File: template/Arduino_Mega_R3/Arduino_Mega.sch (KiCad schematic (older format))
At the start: 7 parts, among them P1 Digital, P2 Power, P3 Analog, P4 Analog, P5 PWM, P6 PWM, P7 Communication

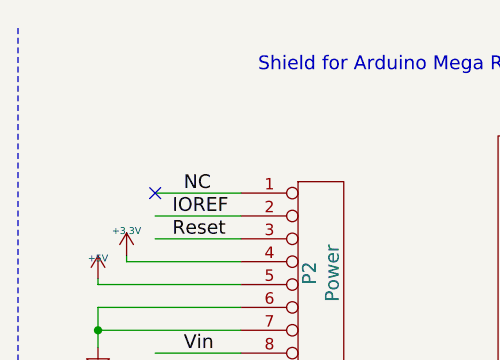
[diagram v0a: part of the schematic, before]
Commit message: correction holes
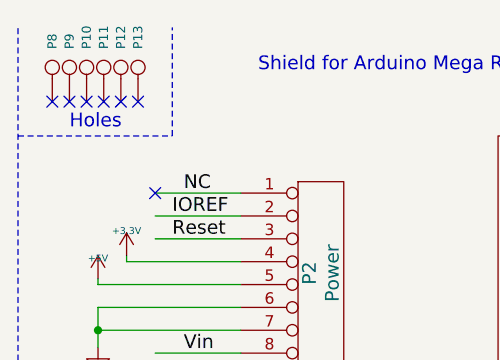
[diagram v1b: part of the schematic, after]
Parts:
- added P10, P11, P12, P13, P8, P9: CONN_1, Connect:1pin, symbol CONN_1
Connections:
- no-connect marks 1 -> 7
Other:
- note added: "Holes"
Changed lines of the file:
@@
 Wire Notes Line
 	7900 6300 7900 475
+$Comp
+L CONN_1 P8
+U 1 1 551BBA20
+P 8050 650
+F 0 "P8" H 8130 650 40  0000 L CNN
+F 1 "CONN_1" H 8050 705 30  0001 C CNN
+F 2 "Connect:1pin" H 8050 650 60  0001 C CNN
+F 3 "" H 8050 650 60  0000 C CNN
+	1    8050 650
+	0    -1   -1   0
+$EndComp
+$Comp
+L CONN_1 P9
+U 1 1 551BBB85
+P 8125 650
+F 0 "P9" H 8205 650 40  0000 L CNN
+F 1 "CONN_1" H 8125 705 30  0001 C CNN
+F 2 "Connect:1pin" H 8125 650 60  0001 C CNN
+F 3 "" H 8125 650 60  0000 C CNN
+	1    8125 650
+	0    -1   -1   0
+$EndComp
+$Comp
+L CONN_1 P10
+U 1 1 551BBBAB
+P 8200 650
+F 0 "P10" H 8280 650 40  0000 L CNN
+F 1 "CONN_1" H 8200 705 30  0001 C CNN
+F 2 "Connect:1pin" H 8200 650 60  0001 C CNN
+F 3 "" H 8200 650 60  0000 C CNN
+	1    8200 650
+	0    -1   -1   0
+$EndComp
+$Comp
+L CONN_1 P11
+U 1 1 551BBBD7
+P 8275 650
+F 0 "P11" H 8355 650 40  0000 L CNN
+F 1 "CONN_1" H 8275 705 30  0001 C CNN
+F 2 "Connect:1pin" H 8275 650 60  0001 C CNN
+F 3 "" H 8275 650 60  0000 C CNN
+	1    8275 650
+	0    -1   -1   0
+$EndComp
+$Comp
+L CONN_1 P12
+U 1 1 551BBC10
+P 8350 650
+F 0 "P12" H 8430 650 40  0000 L CNN
+F 1 "CONN_1" H 8350 705 30  0001 C CNN
+F 2 "Connect:1pin" H 8350 650 60  0001 C CNN
+F 3 "" H 8350 650 60  0000 C CNN
+	1    8350 650
+	0    -1   -1   0
+$EndComp
+$Comp
+L CONN_1 P13
+U 1 1 551BBC3C
+P 8425 650
+F 0 "P13" H 8505 650 40  0000 L CNN
+F 1 "CONN_1" H 8425 705 30  0001 C CNN
+F 2 "Connect:1pin" H 8425 650 60  0001 C CNN
+F 3 "" H 8425 650 60  0000 C CNN
+	1    8425 650
+	0    -1   -1   0
+$EndComp
+NoConn ~ 8050 800
+NoConn ~ 8125 800
+NoConn ~ 8200 800
+NoConn ~ 8275 800
+NoConn ~ 8350 800
+NoConn ~ 8425 800
+Text Notes 8125 925  0    60   ~ 0
+Holes
+Wire Notes Line
+	7900 950  8575 950
+Wire Notes Line
+	8575 950  8575 475
 $EndSCHEMATC

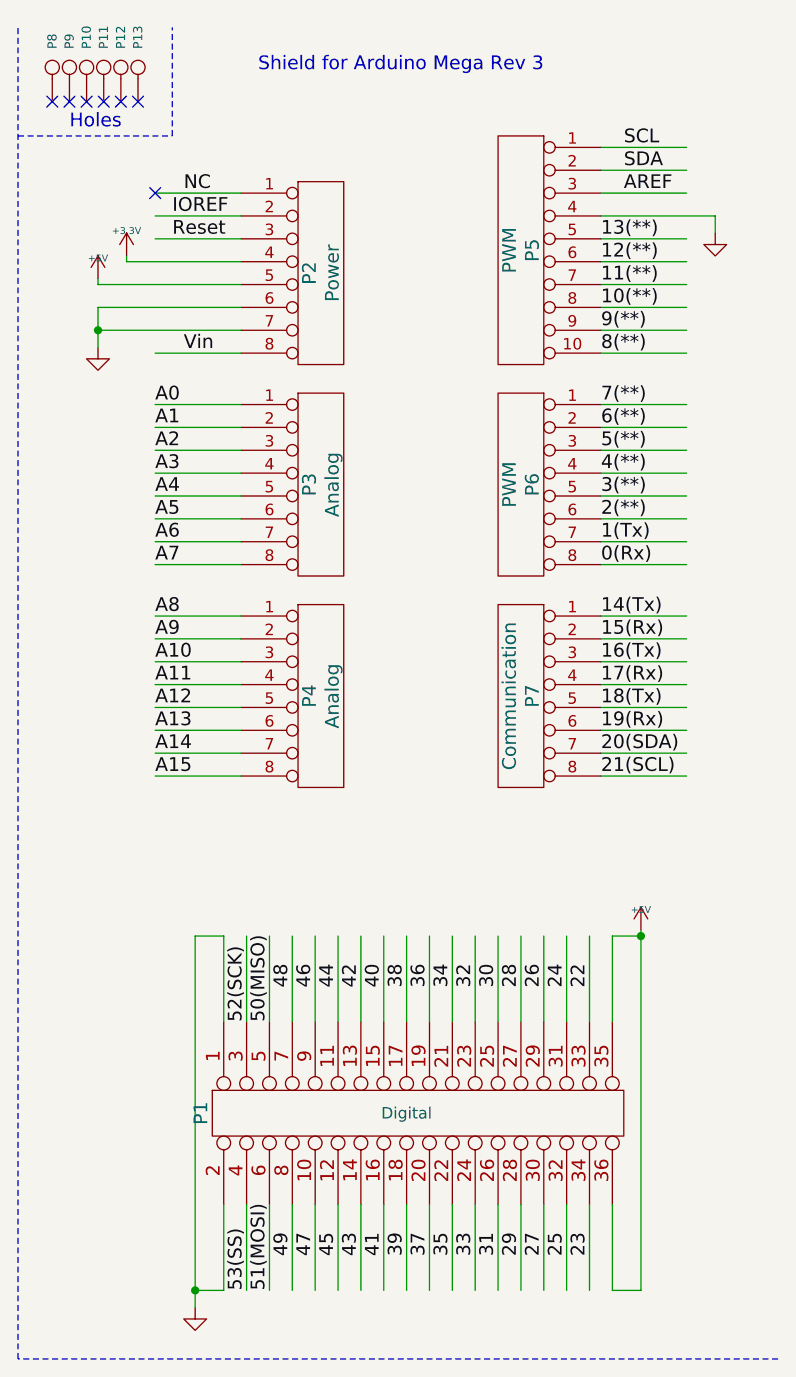
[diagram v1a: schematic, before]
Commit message: Correction schématics
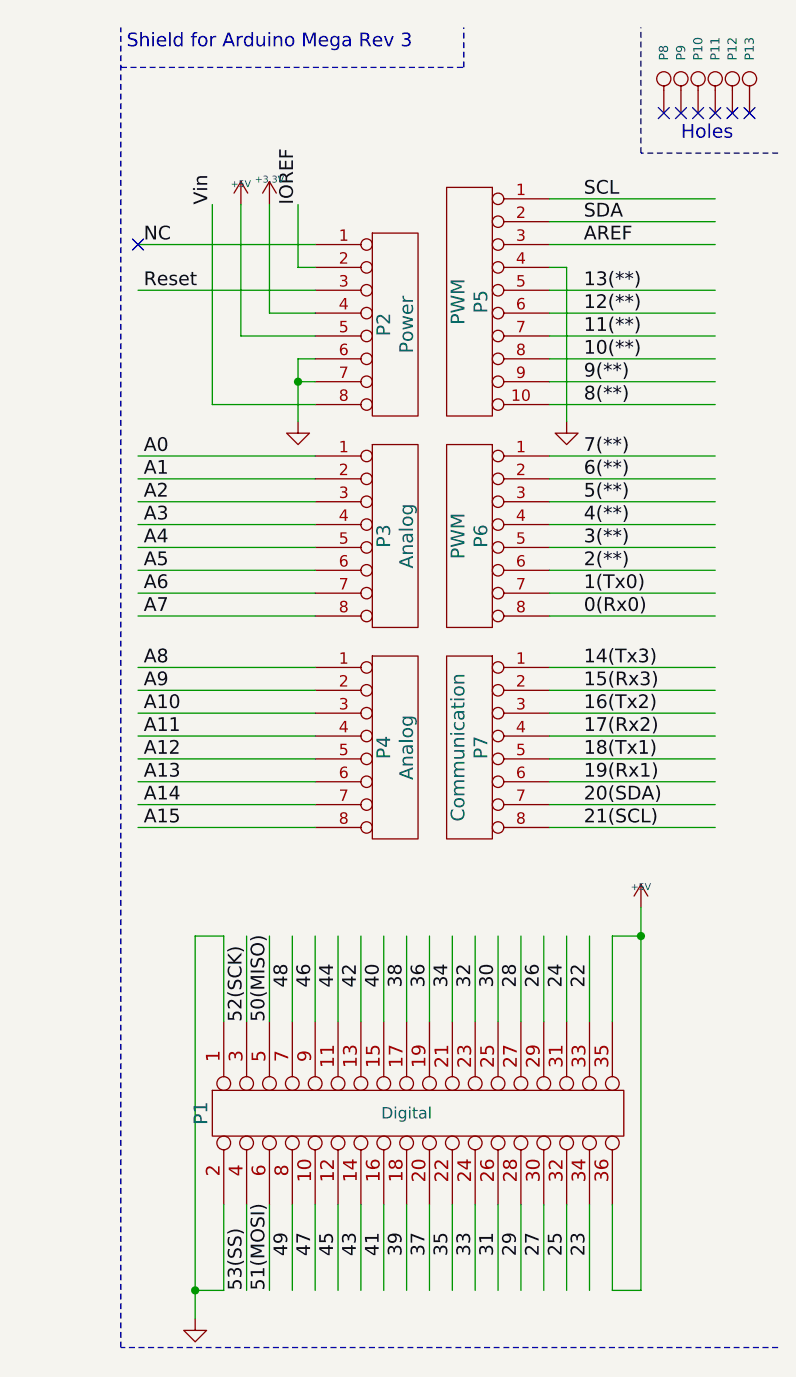
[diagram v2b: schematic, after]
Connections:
- net labels added: 0(Rx0), 1(Tx0), 14(Tx3), 15(Rx3), 16(Tx2), 17(Rx2), 18(Tx1), 19(Rx1)
- net labels removed: 0(Rx), 1(Tx), 14(Tx), 15(Rx), 16(Tx), 17(Rx), 18(Tx), 19(Rx)
- wire segments 96 -> 98
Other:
- moved on the sheet: P10, P11, P12, P13, P2, P3, P4, P5, P6, P7, P8, P9
